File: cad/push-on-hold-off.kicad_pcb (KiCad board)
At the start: 2 copper layers, 11 parts, among them P1 CONN_01X04, P2 CONN_01X04, Q1 IRF7309IPBF, SW1 SW_PUSH_SMALL

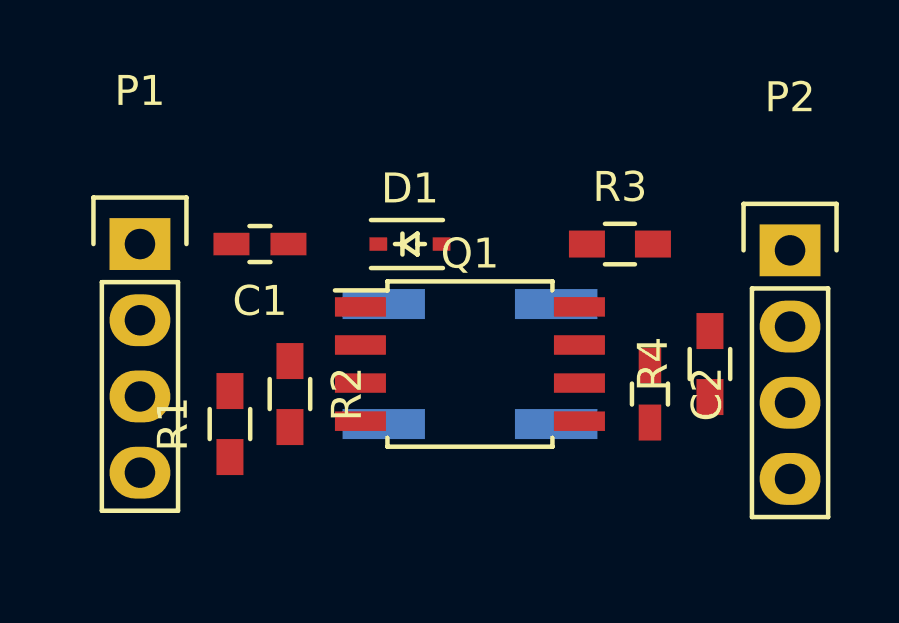
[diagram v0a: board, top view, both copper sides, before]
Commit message: Do some placing and draw outline
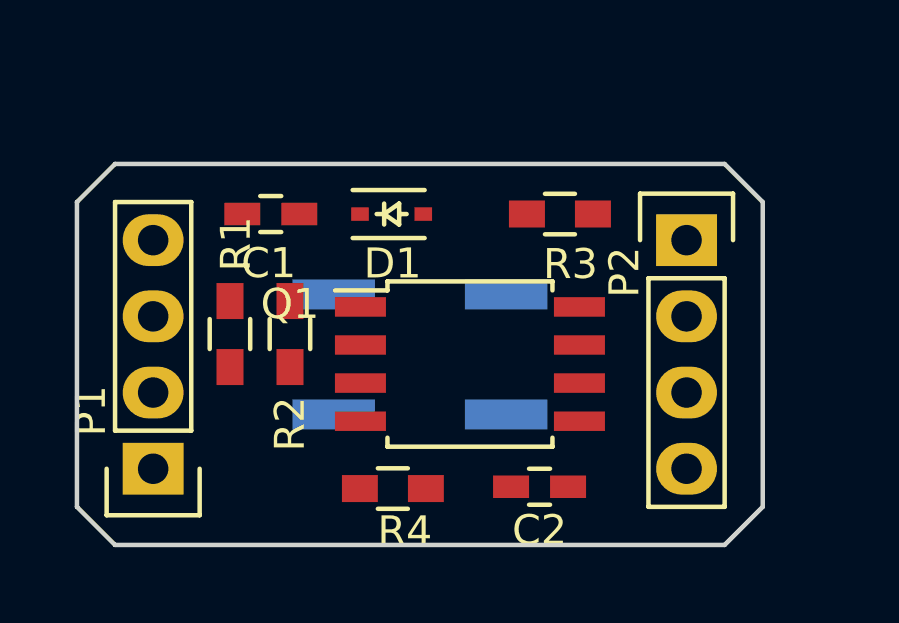
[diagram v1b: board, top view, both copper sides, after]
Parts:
- moved R4 11.4 mm to (226.4, 111.2), turned to 180 degrees
- moved P1 7.50 mm to (218.4, 110.5), turned to 180 degrees
- moved C2 4.81 mm to (231.3, 111.1), turned to 0 degrees
- moved P2 3.47 mm to (236.2, 102.9)
- moved R1 3.00 mm to (221.0, 106.0), turned to 270 degrees
- moved R3 2.24 mm to (232.0, 102.0)
- moved R2 2.00 mm to (223.0, 106.0)
- moved SW1 1.70 mm to (227.3, 106.7)
- moved D1 1.17 mm to (226.4, 102.0)
- moved C1 1.06 mm to (222.4, 102.0)
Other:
- board outline added: 22.9 x 12.7 mm
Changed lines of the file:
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@@
     (links 27)
     (no_connects 27)
-    (area 0 0 0 0)
+    (area 215.824999 100.254999 238.835001 113.105001)
     (thickness 1.6)
-    (drawings 0)
+    (drawings 8)
     (tracks 0)
     (zones 0)
@@
   (layers
     (0 F.Cu signal)
-    (31 B.Cu signal)
+    (31 B.Cu signal hide)
     (32 B.Adhes user)
     (33 F.Adhes user)
@@
     (pad_to_mask_clearance 0.2)
     (aux_axis_origin 0 0)
-    (visible_elements FFFFFF7F)
+    (visible_elements FFFF7F7F)
     (pcbplotparams
       (layerselection 0x00030_80000001)
@@
   )
   (module Capacitors_SMD.pretty:C_0603_HandSoldering (layer F.Cu)
-    (at 222 103 180)
+    (at 222.36 102 180)
     (descr "Capacitor SMD 0603, hand soldering")
     (tags "capacitor 0603")
     (attr smd)
-    (fp_text reference C1 (at 0 -1.9 180) (layer F.SilkS)
-      (effects (font (size 1 1) (thickness 0.15)))
-    )
-    (fp_text value 1uF (at 0 1.9 180) (layer F.Fab)
+    (fp_text reference C1 (at 0.07 -1.64 180) (layer F.SilkS)
+      (effects (font (size 1 1) (thickness 0.15)))
+    )
+    (fp_text value 1uF (at -0.1 -1.51 180) (layer F.Fab)
       (effects (font (size 1 1) (thickness 0.15)))
     )
@@
   )
   (module Diodes_SMD.pretty:SOD-323 (layer F.Cu)
-    (at 227 103)
+    (at 226.39 102)
     (descr SOD-323)
     (tags SOD-323)
     (attr smd)
-    (fp_text reference D1 (at 0 -1.85) (layer F.SilkS)
+    (fp_text reference D1 (at 0.03 1.65) (layer F.SilkS)
       (effects (font (size 1 1) (thickness 0.15)))
     )
@@
     (tags "SOIC 1.27")
     (attr smd)
-    (fp_text reference Q1 (at 0 -3.68) (layer F.SilkS)
-      (effects (font (size 1 1) (thickness 0.15)))
-    )
-    (fp_text value IRF7309IPBF (at 0 3.68) (layer F.Fab)
+    (fp_text reference Q1 (at -6 -2) (layer F.SilkS)
+      (effects (font (size 1 1) (thickness 0.15)))
+    )
+    (fp_text value IRF7309IPBF (at 0.02 3.95) (layer F.Fab)
       (effects (font (size 1 1) (thickness 0.15)))
     )
@@
   )
   (module Resistors_SMD.pretty:R_0603_HandSoldering (layer F.Cu)
-    (at 221 109 90)
+    (at 221 106 270)
     (descr "Resistor SMD 0603, hand soldering")
     (tags "resistor 0603")
     (attr smd)
-    (fp_text reference R1 (at 0 -1.9 90) (layer F.SilkS)
-      (effects (font (size 1 1) (thickness 0.15)))
-    )
-    (fp_text value 10k (at 0 1.9 90) (layer F.Fab)
+    (fp_text reference R1 (at -3 -0.2 270) (layer F.SilkS)
+      (effects (font (size 1 1) (thickness 0.15)))
+    )
+    (fp_text value 10k (at 0 1.9 270) (layer F.Fab)
       (effects (font (size 1 1) (thickness 0.15)))
     )
@@
     (fp_line (start 0.5 0.675) (end -0.5 0.675) (layer F.SilkS) (width 0.15))
     (fp_line (start -0.5 -0.675) (end 0.5 -0.675) (layer F.SilkS) (width 0.15))
-    (pad 1 smd rect (at -1.1 0 90) (size 1.2 0.9) (layers F.Cu F.Paste F.Mask)
+    (pad 1 smd rect (at -1.1 0 270) (size 1.2 0.9) (layers F.Cu F.Paste F.Mask)
       (net 7 /Vin))
-    (pad 2 smd rect (at 1.1 0 90) (size 1.2 0.9) (layers F.Cu F.Paste F.Mask)
+    (pad 2 smd rect (at 1.1 0 270) (size 1.2 0.9) (layers F.Cu F.Paste F.Mask)
       (net 2 /Button))
     (model Resistors_SMD.3dshapes/R_0603_HandSoldering.wrl
@@
   )
   (module Resistors_SMD.pretty:R_0603_HandSoldering (layer F.Cu)
-    (at 223 108 270)
+    (at 223 106 270)
     (descr "Resistor SMD 0603, hand soldering")
     (tags "resistor 0603")
     (attr smd)
-    (fp_text reference R2 (at 0 -1.9 270) (layer F.SilkS)
-      (effects (font (size 1 1) (thickness 0.15)))
-    )
-    (fp_text value 100k (at 0 1.9 270) (layer F.Fab)
+    (fp_text reference R2 (at 3 0 270) (layer F.SilkS)
+      (effects (font (size 1 1) (thickness 0.15)))
+    )
+    (fp_text value 100k (at 0.91 1.77 270) (layer F.Fab)
       (effects (font (size 1 1) (thickness 0.15)))
     )
@@
   )
   (module Resistors_SMD.pretty:R_0603_HandSoldering (layer F.Cu)
-    (at 234 103)
+    (at 232 102)
     (descr "Resistor SMD 0603, hand soldering")
     (tags "resistor 0603")
     (attr smd)
-    (fp_text reference R3 (at 0 -1.9) (layer F.SilkS)
+    (fp_text reference R3 (at 0.35 1.67) (layer F.SilkS)
       (effects (font (size 1 1) (thickness 0.15)))
     )
@@
   )
   (module Resistors_SMD.pretty:R_0603_HandSoldering (layer F.Cu)
-    (at 237 107 90)
+    (at 226.43 111.15 180)
     (descr "Resistor SMD 0603, hand soldering")
     (tags "resistor 0603")
     (attr smd)
-    (fp_text reference R4 (at 0 -1.9 90) (layer F.SilkS)
-      (effects (font (size 1 1) (thickness 0.15)))
-    )
-    (fp_text value 100k (at 0 1.9 90) (layer F.Fab)
+    (fp_text reference R4 (at -0.4 -1.43 180) (layer F.SilkS)
+      (effects (font (size 1 1) (thickness 0.15)))
+    )
+    (fp_text value 100k (at 0 1.9 180) (layer F.Fab)
       (effects (font (size 1 1) (thickness 0.15)))
     )
@@
     (fp_line (start 0.5 0.675) (end -0.5 0.675) (layer F.SilkS) (width 0.15))
     (fp_line (start -0.5 -0.675) (end 0.5 -0.675) (layer F.SilkS) (width 0.15))
-    (pad 1 smd rect (at -1.1 0 90) (size 1.2 0.9) (layers F.Cu F.Paste F.Mask)
+    (pad 1 smd rect (at -1.1 0 180) (size 1.2 0.9) (layers F.Cu F.Paste F.Mask)
       (net 4 /Vout))
-    (pad 2 smd rect (at 1.1 0 90) (size 1.2 0.9) (layers F.Cu F.Paste F.Mask)
+    (pad 2 smd rect (at 1.1 0 180) (size 1.2 0.9) (layers F.Cu F.Paste F.Mask)
       (net 5 "Net-(D1-Pad2)"))
     (model Resistors_SMD.3dshapes/R_0603_HandSoldering.wrl
@@
   )
   (module Buttons_Switches_SMD.pretty:SW_SPST_EVPBF (layer B.Cu)
-    (at 229 107)
+    (at 227.33 106.68)
     (descr "Light Touch Switch")
     (attr smd)
@@
   )
   (module Pin_Headers.pretty:Pin_Header_Straight_1x04 (layer F.Cu)
-    (at 218 103)
+    (at 218.44 110.49 180)
     (descr "Through hole pin header")
     (tags "pin header")
-    (fp_text reference P1 (at 0 -5.1) (layer F.SilkS)
-      (effects (font (size 1 1) (thickness 0.15)))
-    )
-    (fp_text value CONN_01X04 (at 0 -3.1) (layer F.Fab)
+    (fp_text reference P1 (at 2.07 1.93 270) (layer F.SilkS)
+      (effects (font (size 1 1) (thickness 0.15)))
+    )
+    (fp_text value CONN_01X04 (at 0 -3.1 180) (layer F.Fab)
       (effects (font (size 1 1) (thickness 0.15)))
     )
@@
     (fp_line (start -1.55 0) (end -1.55 -1.55) (layer F.SilkS) (width 0.15))
     (fp_line (start -1.55 -1.55) (end 1.55 -1.55) (layer F.SilkS) (width 0.15))
-    (pad 1 thru_hole rect (at 0 0) (size 2.032 1.7272) (drill 1.016) (layers *.Cu *.Mask F.SilkS)
-      (net 6 GND))
-    (pad 2 thru_hole oval (at 0 2.54) (size 2.032 1.7272) (drill 1.016) (layers *.Cu *.Mask F.SilkS)
-      (net 6 GND))
-    (pad 3 thru_hole oval (at 0 5.08) (size 2.032 1.7272) (drill 1.016) (layers *.Cu *.Mask F.SilkS)
-      (net 2 /Button))
-    (pad 4 thru_hole oval (at 0 7.62) (size 2.032 1.7272) (drill 1.016) (layers *.Cu *.Mask F.SilkS)
+    (pad 1 thru_hole rect (at 0 0 180) (size 2.032 1.7272) (drill 1.016) (layers *.Cu *.Mask F.SilkS)
+      (net 6 GND))
+    (pad 2 thru_hole oval (at 0 2.54 180) (size 2.032 1.7272) (drill 1.016) (layers *.Cu *.Mask F.SilkS)
+      (net 6 GND))
+    (pad 3 thru_hole oval (at 0 5.08 180) (size 2.032 1.7272) (drill 1.016) (layers *.Cu *.Mask F.SilkS)
+      (net 2 /Button))
+    (pad 4 thru_hole oval (at 0 7.62 180) (size 2.032 1.7272) (drill 1.016) (layers *.Cu *.Mask F.SilkS)
       (net 7 /Vin))
     (model Pin_Headers.3dshapes/Pin_Header_Straight_1x04.wrl
@@
   )
   (module Pin_Headers.pretty:Pin_Header_Straight_1x04 (layer F.Cu)
-    (at 239.67 103.21)
+    (at 236.22 102.87)
     (descr "Through hole pin header")
     (tags "pin header")
-    (fp_text reference P2 (at 0 -5.1) (layer F.SilkS)
+    (fp_text reference P2 (at -2.07 1.07 90) (layer F.SilkS)
       (effects (font (size 1 1) (thickness 0.15)))
     )
@@
   )
   (module Capacitors_SMD.pretty:C_0603_HandSoldering (layer F.Cu)
-    (at 235 108 270)
+    (at 231.32 111.09)
     (descr "Capacitor SMD 0603, hand soldering")
     (tags "capacitor 0603")
     (attr smd)
-    (fp_text reference C2 (at 0 -1.9 270) (layer F.SilkS)
-      (effects (font (size 1 1) (thickness 0.15)))
-    )
-    (fp_text value 10uF (at 0 1.9 270) (layer F.Fab)
+    (fp_text reference C2 (at 0 1.45) (layer F.SilkS)
+      (effects (font (size 1 1) (thickness 0.15)))
+    )
+    (fp_text value 10uF (at 0 1.9) (layer F.Fab)
       (effects (font (size 1 1) (thickness 0.15)))
     )
@@
     (fp_line (start -0.35 -0.6) (end 0.35 -0.6) (layer F.SilkS) (width 0.15))
     (fp_line (start 0.35 0.6) (end -0.35 0.6) (layer F.SilkS) (width 0.15))
-    (pad 1 smd rect (at -0.95 0 270) (size 1.2 0.75) (layers F.Cu F.Paste F.Mask)
+    (pad 1 smd rect (at -0.95 0) (size 1.2 0.75) (layers F.Cu F.Paste F.Mask)
       (net 3 "Net-(C2-Pad1)"))
-    (pad 2 smd rect (at 0.95 0 270) (size 1.2 0.75) (layers F.Cu F.Paste F.Mask)
+    (pad 2 smd rect (at 0.95 0) (size 1.2 0.75) (layers F.Cu F.Paste F.Mask)
       (net 4 /Vout))
     (model Capacitors_SMD.3dshapes/C_0603_HandSoldering.wrl
@@
     )
   )
+  (gr_line (start 237.49 100.33) (end 217.17 100.33) (angle 90) (layer Edge.Cuts) (width 0.15))
+  (gr_line (start 238.76 101.6) (end 237.49 100.33) (angle 90) (layer Edge.Cuts) (width 0.15))
+  (gr_line (start 238.76 111.76) (end 238.76 101.6) (angle 90) (layer Edge.Cuts) (width 0.15))
+  (gr_line (start 237.49 113.03) (end 238.76 111.76) (angle 90) (layer Edge.Cuts) (width 0.15))
+  (gr_line (start 217.17 113.03) (end 237.49 113.03) (angle 90) (layer Edge.Cuts) (width 0.15))
+  (gr_line (start 215.9 111.76) (end 217.17 113.03) (angle 90) (layer Edge.Cuts) (width 0.15))
+  (gr_line (start 215.9 101.6) (end 215.9 111.76) (angle 90) (layer Edge.Cuts) (width 0.15))
+  (gr_line (start 217.17 100.33) (end 215.9 101.6) (angle 90) (layer Edge.Cuts) (width 0.15))
 )
